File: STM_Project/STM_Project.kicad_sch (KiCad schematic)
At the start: 24 parts, among them J1 Conn_01x04_Pin, J2 USB_B_Micro, SW1 SW_SPDT, U1 STM32F103C8Tx, U2 AMS1117-3.3, Y1 16MHz

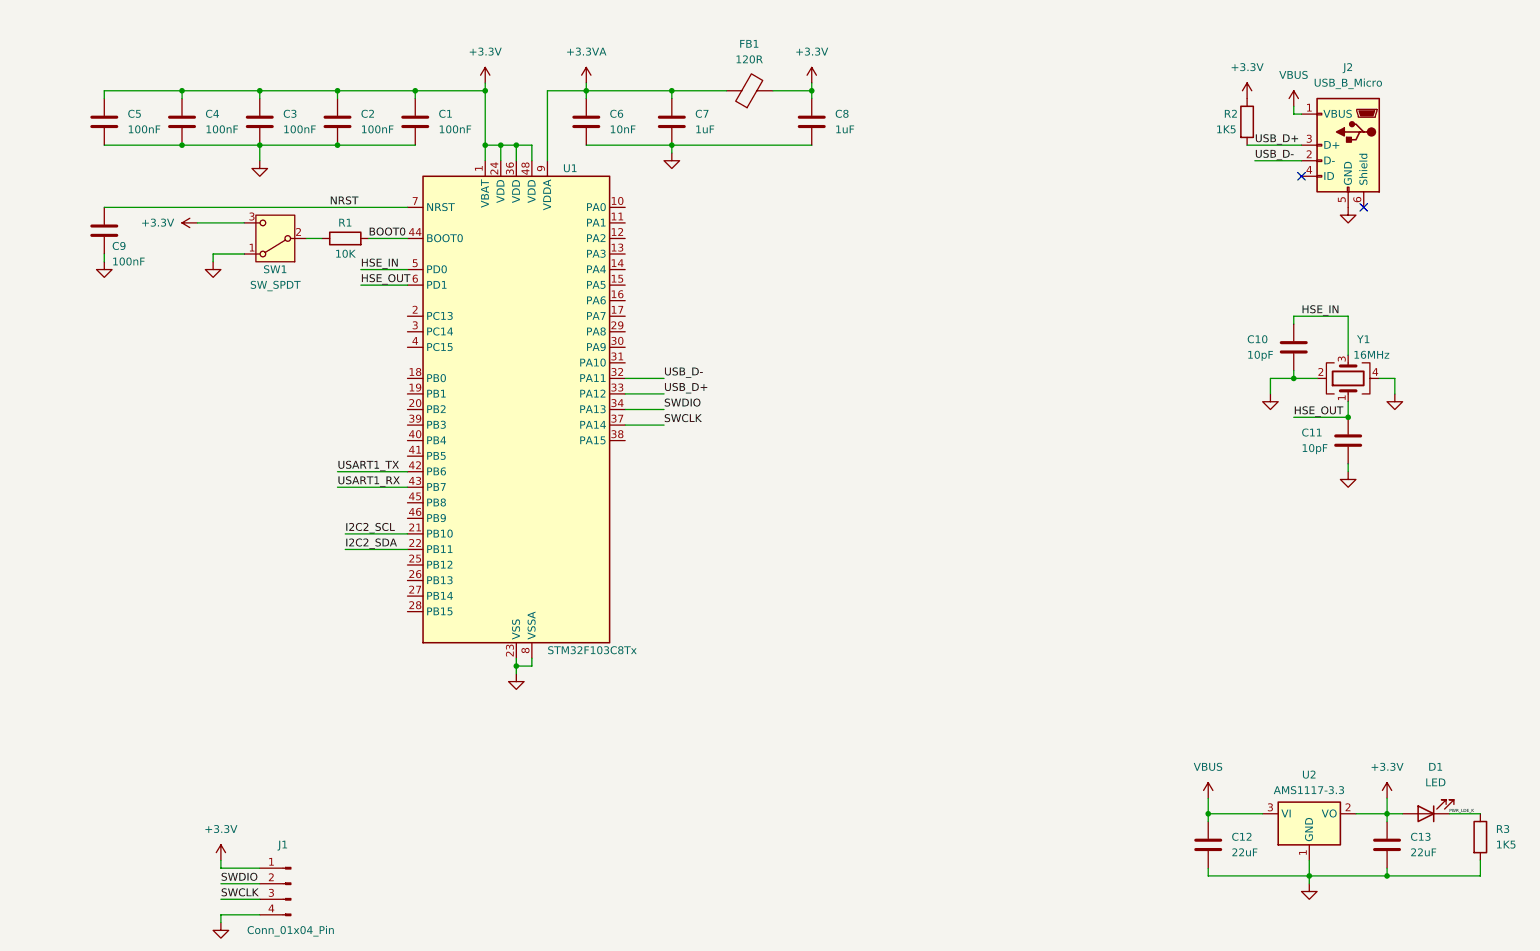
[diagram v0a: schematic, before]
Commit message: Finish SCH
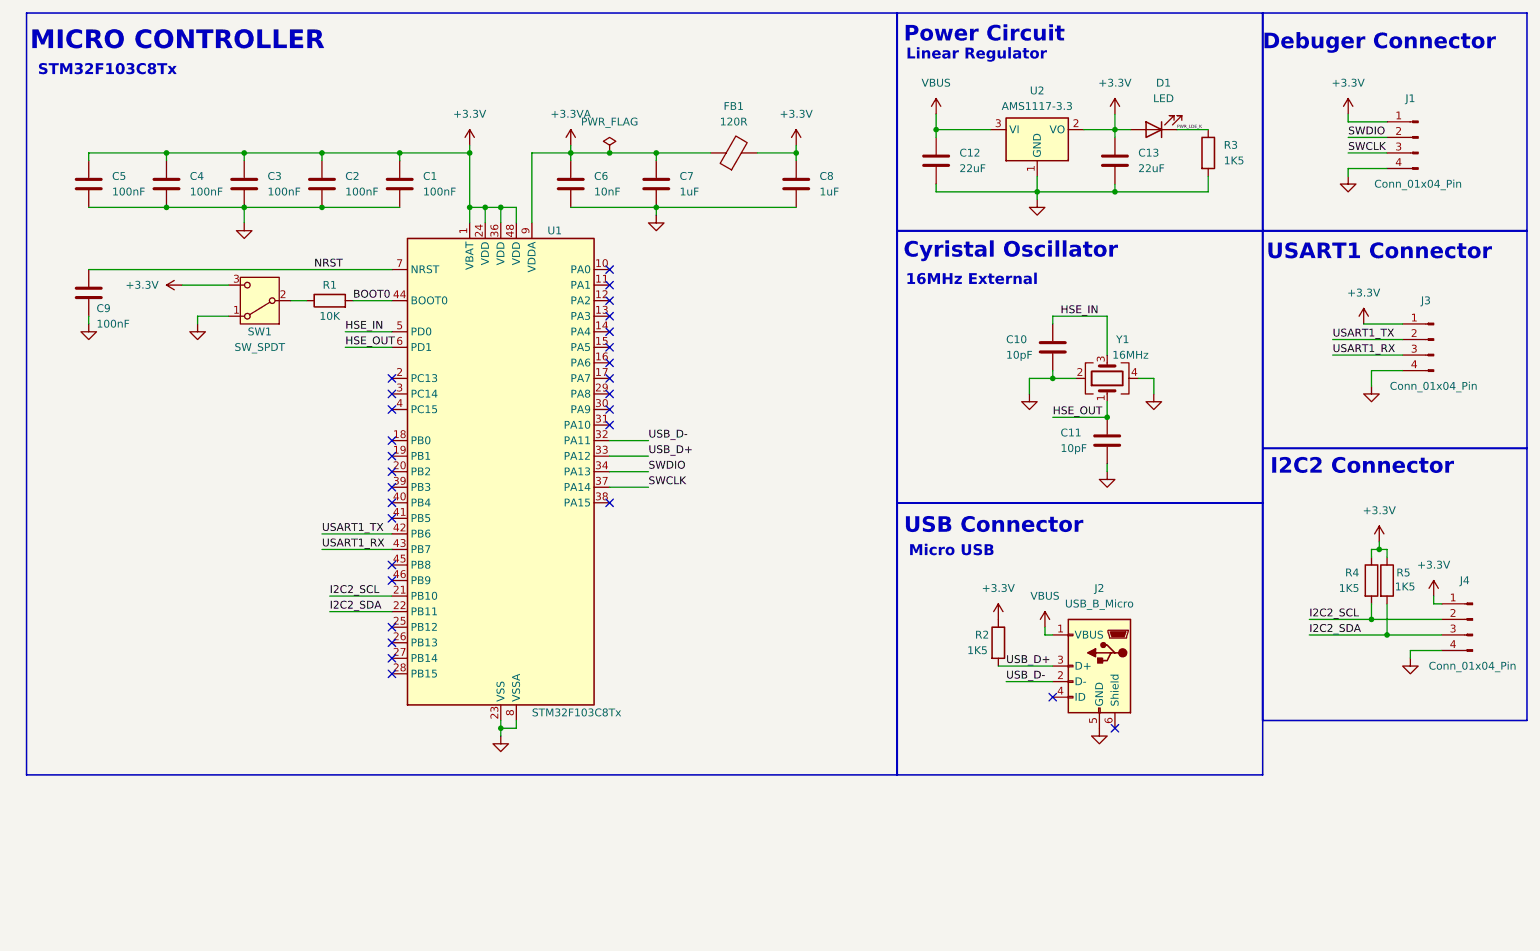
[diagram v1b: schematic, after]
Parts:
- added J3, J4: Conn_01x04_Pin, Connector_PinHeader_2.54mm:PinHeader_1x04_P2.54mm_Vertical, symbol Connector:Conn_01x04_Pin
- added R4, R5: 1K5, Resistor_SMD:R_0603_1608Metric, symbol Device:R
- C1, C10, C11, C2, C3, C4, C5, C6, C9: footprint (none) -> Capacitor_SMD:C_0603_1608Metric
- C12, C13, C7, C8: footprint (none) -> Capacitor_SMD:C_0805_2012Metric
- D1: footprint (none) -> LED_SMD:LED_0603_1608Metric
- FB1: footprint (none) -> Inductor_SMD:L_0603_1608Metric
- J1: footprint (none) -> Connector_PinHeader_2.54mm:PinHeader_1x04_P2.54mm_Vertical
- J2: footprint (none) -> Connector_USB:USB_Micro-B_Technik_TWP-4002D-H3
- R1, R2, R3: footprint (none) -> Resistor_SMD:R_0603_1608Metric
- SW1: footprint (none) -> Button_Switch_THT:SW_E-Switch_EG1224_SPDT_Angled
- Y1: footprint (none) -> Crystal:Crystal_SMD_3225-4Pin_3.2x2.5mm
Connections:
- net +3.3V: now also J3.1 (Pin_1), J4.1 (Pin_1), R4.1, R5.1
- net GND: now also J3.4 (Pin_4), J4.4 (Pin_4)
- net I2C2_SCL: now also J4.2 (Pin_2), R4.2
- net I2C2_SDA: now also J4.3 (Pin_3), R5.2
- net USART1_RX: now also J3.3 (Pin_3)
- net USART1_TX: now also J3.2 (Pin_2)
- no-connect marks 2 -> 29
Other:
- note added: "16MHz External"
- note added: "Cyristal Oscillator"
- note added: "Debuger Connector"
- note added: "I2C2 Connector"
- note added: "Linear Regulator"
- note added: "MICRO CONTROLLER"
- note added: "Micro USB"
- note added: "Power Circuit"
- note added: "STM32F103C8Tx"
- note added: "USART1 Connector"
- note added: "USB Connector"
- moved on the sheet: C1, C10, C11, C12, C13, C2, C3, C4, C5, C6, C7, C8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
